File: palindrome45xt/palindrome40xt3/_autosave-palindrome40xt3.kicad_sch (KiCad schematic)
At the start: 110 parts, among them J1 Conn_01x02_Socket, Q1 Q_NMOS_GDS, Q3 TIP120, U1 RP2040_Zero

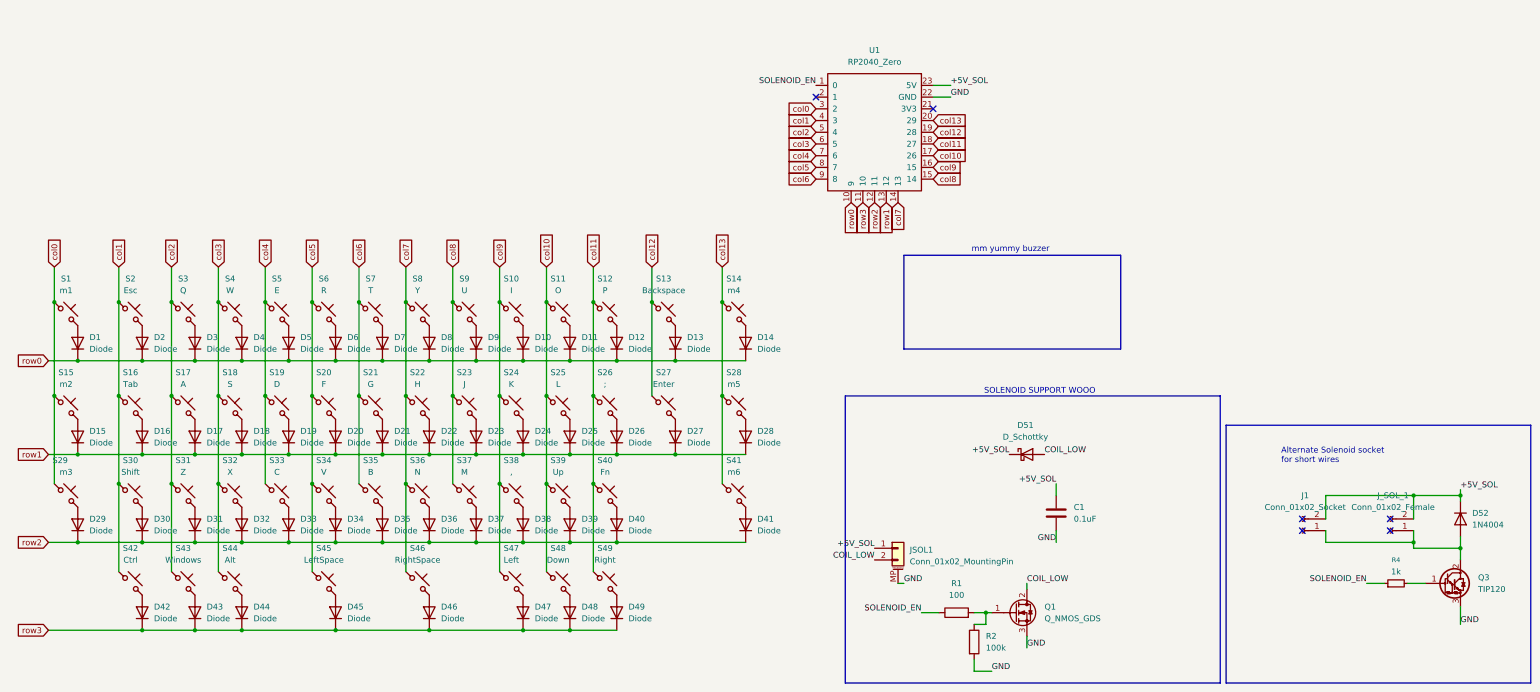
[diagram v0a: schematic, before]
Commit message: disaster here
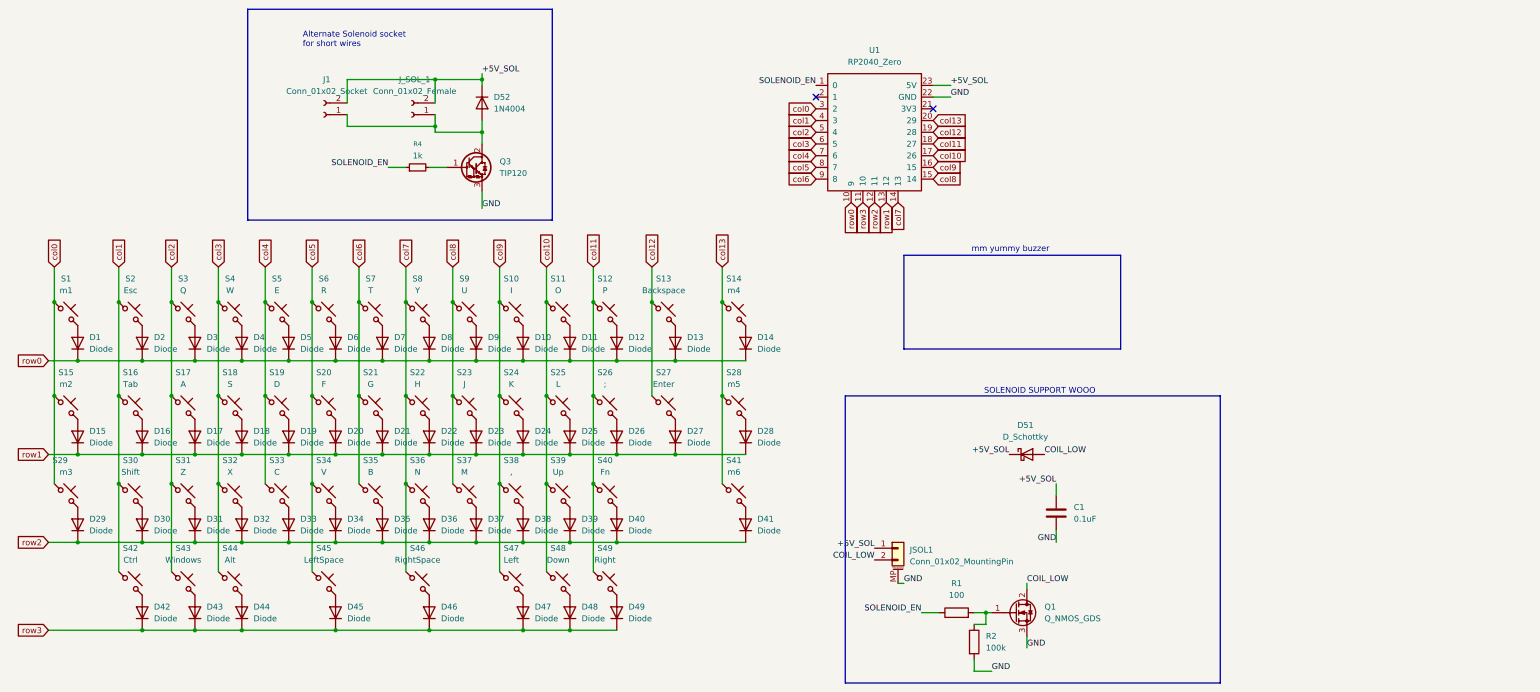
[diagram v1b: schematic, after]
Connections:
- no-connect marks 6 -> 2
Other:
- moved on the sheet: D52, J1, J_SOL_1, Q3, R4
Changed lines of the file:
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@@
 	(paper "A4")
 	(rectangle
-		(start 274.32 106.68)
-		(end 340.36 162.56)
+		(start 62.23 16.51)
+		(end 128.27 62.23)
 		(stroke
 			(width 0)
@@
 	(text "Alternate Solenoid socket \nfor short wires"
 		(exclude_from_sim no)
-		(at 286.258 115.062 0)
+		(at 74.168 24.892 0)
 		(effects
 			(font
@@
 	)
 	(junction
-		(at 325.12 133.35)
+		(at 113.03 43.18)
 		(diameter 0)
 		(color 0 0 0 0)
@@
 	)
 	(junction
-		(at 314.96 132.08)
+		(at 102.87 41.91)
 		(diameter 0)
 		(color 0 0 0 0)
@@
 	)
 	(junction
-		(at 314.96 121.92)
+		(at 102.87 31.75)
 		(diameter 0)
 		(color 0 0 0 0)
@@
 	)
 	(junction
-		(at 325.12 121.92)
+		(at 113.03 31.75)
 		(diameter 0)
 		(color 0 0 0 0)
@@
 	)
 	(no_connect
-		(at 309.88 129.54)
-	)
-	(no_connect
-		(at 290.83 127)
-	)
-	(no_connect
-		(at 290.83 129.54)
-	)
-	(no_connect
 		(at 210.82 38.1)
 	)
@@
 		(at 185.42 35.56)
 	)
-	(no_connect
-		(at 309.88 127)
-	)
 	(wire
 		(pts
@@
 	(wire
 		(pts
-			(xy 314.96 133.35) (xy 325.12 133.35)
+			(xy 102.87 43.18) (xy 113.03 43.18)
 		)
 		(stroke
@@
 	(wire
 		(pts
-			(xy 314.96 132.08) (xy 314.96 129.54)
+			(xy 102.87 41.91) (xy 102.87 39.37)
 		)
 		(stroke
@@
 	(wire
 		(pts
-			(xy 295.91 129.54) (xy 295.91 132.08)
+			(xy 83.82 39.37) (xy 83.82 41.91)
 		)
 		(stroke
@@
 	(wire
 		(pts
-			(xy 325.12 121.92) (xy 325.12 123.19)
+			(xy 113.03 31.75) (xy 113.03 33.02)
 		)
 		(stroke
@@
 	(wire
 		(pts
-			(xy 295.91 132.08) (xy 314.96 132.08)
+			(xy 83.82 41.91) (xy 102.87 41.91)
 		)
 		(stroke
@@
 	(wire
 		(pts
-			(xy 325.12 120.65) (xy 325.12 121.92)
+			(xy 113.03 30.48) (xy 113.03 31.75)
 		)
 		(stroke
@@
 	(wire
 		(pts
-			(xy 314.96 121.92) (xy 314.96 127)
+			(xy 102.87 31.75) (xy 102.87 36.83)
 		)
 		(stroke
@@
 	(wire
 		(pts
-			(xy 308.61 140.97) (xy 304.8 140.97)
+			(xy 96.52 50.8) (xy 92.71 50.8)
 		)
 		(stroke
@@
 	(wire
 		(pts
-			(xy 314.96 121.92) (xy 325.12 121.92)
+			(xy 102.87 31.75) (xy 113.03 31.75)
 		)
 		(stroke
@@
 	(wire
 		(pts
-			(xy 325.12 130.81) (xy 325.12 133.35)
+			(xy 113.03 40.64) (xy 113.03 43.18)
 		)
 		(stroke
@@
 	(wire
 		(pts
-			(xy 314.96 133.35) (xy 314.96 132.08)
+			(xy 102.87 43.18) (xy 102.87 41.91)
 		)
 		(stroke
@@
 	(wire
 		(pts
-			(xy 295.91 127) (xy 295.91 121.92)
+			(xy 83.82 36.83) (xy 83.82 31.75)
 		)
 		(stroke
@@
 	(wire
 		(pts
-			(xy 295.91 121.92) (xy 314.96 121.92)
+			(xy 83.82 31.75) (xy 102.87 31.75)
 		)
 		(stroke
@@
 	(wire
 		(pts
-			(xy 325.12 149.86) (xy 325.12 146.05)
+			(xy 113.03 59.69) (xy 113.03 55.88)
 		)
 		(stroke
@@
 	(wire
 		(pts
-			(xy 313.69 140.97) (xy 317.5 140.97)
+			(xy 101.6 50.8) (xy 105.41 50.8)
 		)
 		(stroke
@@
 	(wire
 		(pts
-			(xy 325.12 133.35) (xy 325.12 135.89)
+			(xy 113.03 43.18) (xy 113.03 45.72)
 		)
 		(stroke
@@
 	)
 	(label "SOLENOID_EN"
-		(at 304.8 140.97 180)
+		(at 92.71 50.8 180)
 		(fields_autoplaced yes)
 		(effects
@@
 		)
 		(property "SOLENOID_EN" ""
-			(at 304.8 142.24 0)
+			(at 92.71 52.07 0)
 			(effects
 				(font
@@
 	)
 	(label "+5V_SOL"
-		(at 325.12 120.65 0)
+		(at 113.03 30.48 0)
 		(fields_autoplaced yes)
 		(effects
@@
 		)
 		(property "+12V_SOL" ""
-			(at 325.12 121.92 0)
+			(at 113.03 31.75 0)
 			(effects
 				(font
@@
 	)
 	(label "GND"
-		(at 325.12 149.86 0)
+		(at 113.03 59.69 0)
 		(fields_autoplaced yes)
 		(effects
@@
 		)
 		(property "GND" ""
-			(at 325.12 151.13 0)
+			(at 113.03 60.96 0)
 			(effects
 				(font
@@
 	(symbol
 		(lib_id "Transistor_BJT:TIP120")
-		(at 322.58 140.97 0)
+		(at 110.49 50.8 0)
 		(unit 1)
 		(exclude_from_sim no)
@@
 		(fields_autoplaced yes)
 		(property "Reference" "Q3"
-			(at 328.93 139.7 0)
+			(at 116.84 49.53 0)
 			(effects
 				(font
@@
 		)
 		(property "Value" "TIP120"
-			(at 328.93 142.24 0)
+			(at 116.84 52.07 0)
 			(effects
 				(font
@@
 		)
 		(property "Footprint" "ergodonk_simple_zero:TO-220-3_Horizontal_TabDown_ergodonk_simple_zero"
-			(at 327.66 142.875 0)
+			(at 115.57 52.705 0)
 			(effects
 				(font
@@
 		)
 		(property "Datasheet" "https://www.onsemi.com/pub/Collateral/TIP120-D.PDF"
-			(at 322.58 140.97 0)
+			(at 110.49 50.8 0)
 			(effects
 				(font
@@
 		)
 		(property "Description" "5A Ic, 60V Vce, Silicon Darlington Power NPN Transistor, TO-220"
-			(at 322.58 140.97 0)
+			(at 110.49 50.8 0)
 			(effects
 				(font
@@
 	(symbol
 		(lib_id "Connector:Conn_01x02_Socket")
-		(at 290.83 129.54 180)
+		(at 78.74 39.37 180)
 		(unit 1)
 		(exclude_from_sim no)
@@
 		(fields_autoplaced yes)
 		(property "Reference" "J1"
-			(at 291.465 121.92 0)
+			(at 79.375 31.75 0)
 			(effects
 				(font
@@
 		)
 		(property "Value" "Conn_01x02_Socket"
-			(at 291.465 124.46 0)
+			(at 79.375 34.29 0)
 			(effects
 				(font
@@
 		)
 		(property "Footprint" "ergodonk_simple_zero:PinHeader_1x02_P2.54mm_Vertical"
-			(at 290.83 129.54 0)
+			(at 78.74 39.37 0)
 			(effects
 				(font
@@
 		)
 		(property "Datasheet" "~"
-			(at 290.83 129.54 0)
+			(at 78.74 39.37 0)
 			(effects
 				(font
@@
 		)
 		(property "Description" "Generic connector, single row, 01x02, script generated"
-			(at 290.83 129.54 0)
+			(at 78.74 39.37 0)
 			(effects
 				(font
@@
 	(symbol
 		(lib_id "Connector:Conn_01x02_Socket")
-		(at 309.88 129.54 180)
+		(at 97.79 39.37 180)
 		(unit 1)
 		(exclude_from_sim no)
@@
 		(on_board yes)
 		(dnp no)
-		(fields_autoplaced yes)
 		(property "Reference" "J_SOL_1"
-			(at 310.515 121.92 0)
+			(at 98.425 31.75 0)
 			(effects
 				(font
@@
 		)
 		(property "Value" "Conn_01x02_Female"
-			(at 310.515 124.46 0)
+			(at 98.425 34.29 0)
 			(effects
 				(font
@@
 		)
 		(property "Footprint" "ergodonk_simple_zero:PinHeader_1x02_P2.54mm_Vertical"
-			(at 309.88 129.54 0)
+			(at 97.79 39.37 0)
 			(effects
 				(font
@@
 		)
 		(property "Datasheet" "~"
-			(at 309.88 129.54 0)
+			(at 97.79 39.37 0)
 			(effects
 				(font
@@
 		)
 		(property "Description" "Generic connector, single row, 01x02, script generated"
-			(at 309.88 129.54 0)
+			(at 97.79 39.37 0)
 			(effects
 				(font
@@
 		(lib_name "R_Small_1")
 		(lib_id "Device:R_Small")
-		(at 311.15 140.97 90)
+		(at 99.06 50.8 90)
 		(unit 1)
 		(exclude_from_sim no)
@@
 		(fields_autoplaced yes)
 		(property "Reference" "R4"
-			(at 311.15 135.89 90)
+			(at 99.06 45.72 90)
 			(effects
 				(font
@@
 		)
 		(property "Value" "1k"
-			(at 311.15 138.43 90)
+			(at 99.06 48.26 90)
 			(effects
 				(font
@@
 		)
 		(property "Footprint" "ergodonk_simple_zero:R_Axial_DIN0309_L9.0mm_D3.2mm_P12.70mm_Horizontal"
-			(at 311.15 140.97 0)
+			(at 99.06 50.8 0)
 			(effects
 				(font
@@
 		)
 		(property "Datasheet" "~"
-			(at 311.15 140.97 0)
+			(at 99.06 50.8 0)
 			(effects
 				(font
@@
 		)
 		(property "Description" "Resistor, small symbol"
-			(at 311.15 140.97 0)
+			(at 99.06 50.8 0)
 			(effects
 				(font
@@
 	(symbol
 		(lib_id "Diode:1N4004")
-		(at 325.12 127 270)
+		(at 113.03 36.83 270)
 		(unit 1)
 		(exclude_from_sim no)
@@
 		(fields_autoplaced yes)
 		(property "Reference" "D52"
-			(at 327.66 125.73 90)
+			(at 115.57 35.56 90)
 			(effects
 				(font
@@
 		)
 		(property "Value" "1N4004"
-			(at 327.66 128.27 90)
+			(at 115.57 38.1 90)
 			(effects
 				(font
@@
 		)
 		(property "Footprint" "ergodonk_simple_zero:D_DO-41_SOD81_P10.16mm_Horizontal"
-			(at 320.675 127 0)
+			(at 108.585 36.83 0)
 			(effects
 				(font
@@
 		)
 		(property "Datasheet" "http://www.vishay.com/docs/88503/1n4001.pdf"
-			(at 325.12 127 0)
+			(at 113.03 36.83 0)
 			(effects
 				(font
@@
 		)
 		(property "Description" ""
-			(at 325.12 127 0)
+			(at 113.03 36.83 0)
 			(effects
 				(font
@@
 		)
 		(property "Sim.Device" "D"
-			(at 325.12 127 0)
+			(at 113.03 36.83 0)
 			(effects
 				(font
@@
 		)
 		(property "Sim.Pins" "1=K 2=A"
-			(at 325.12 127 0)
+			(at 113.03 36.83 0)
 			(effects
 				(font
